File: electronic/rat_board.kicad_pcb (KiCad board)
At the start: 2 copper layers, 44.5 x 49.5 mm, 52 parts, among them P1 FRONT_LEFT_IR, P2 SIDE_LEFT_IR, P3 SIDE_RIGHT_IR, P4 FRONT_RIGHT_IR, P5 LEFT_MOTOR, P6 RIGHT_MOTOR, P7 JTAG, SW1 SW_PUSH_SMALL_H, SW2 SWITCH_INV, SW3 SELECT_BUTTON, SW4 START_BUTTON, U1 TR05S3V3, U2 TB6612FNG, U3 STM32F103C8T6, Y1 32.768kHz, Y2 8MHz

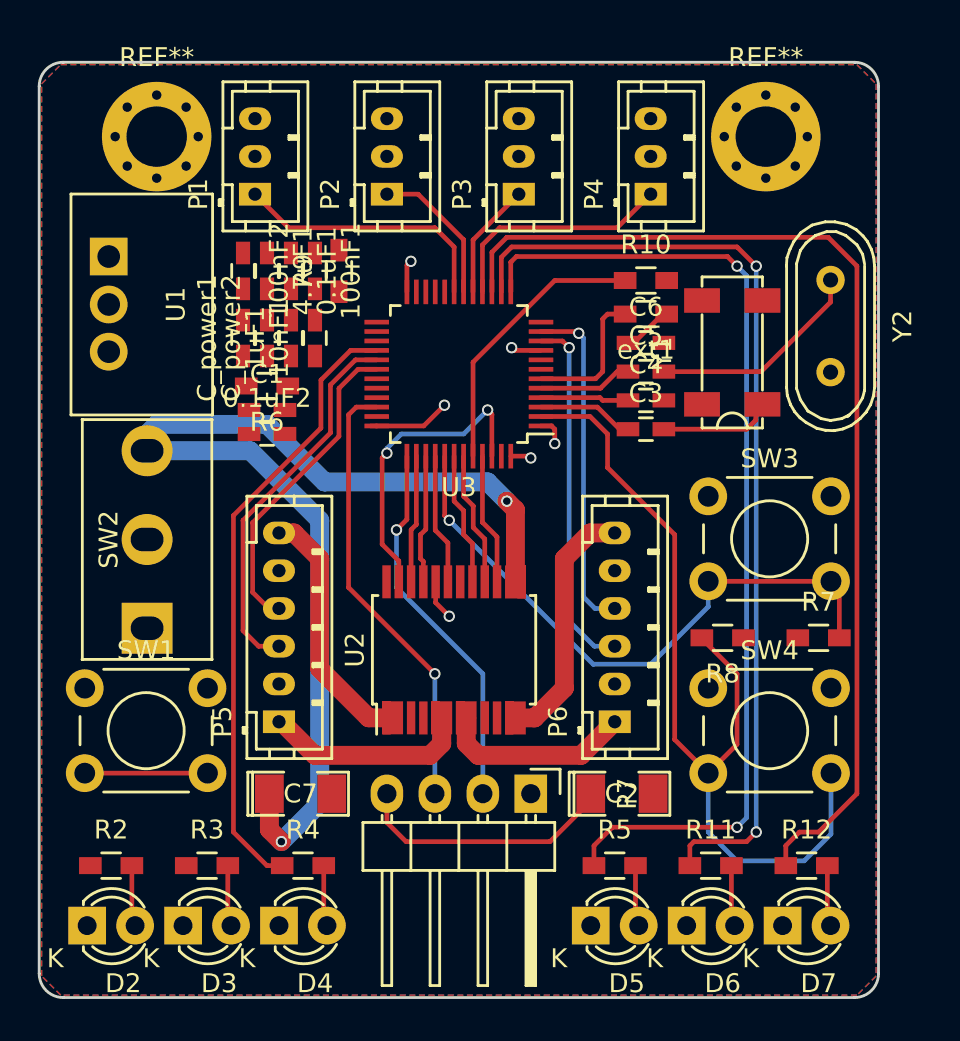
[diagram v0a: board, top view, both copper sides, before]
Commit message: updated pcb
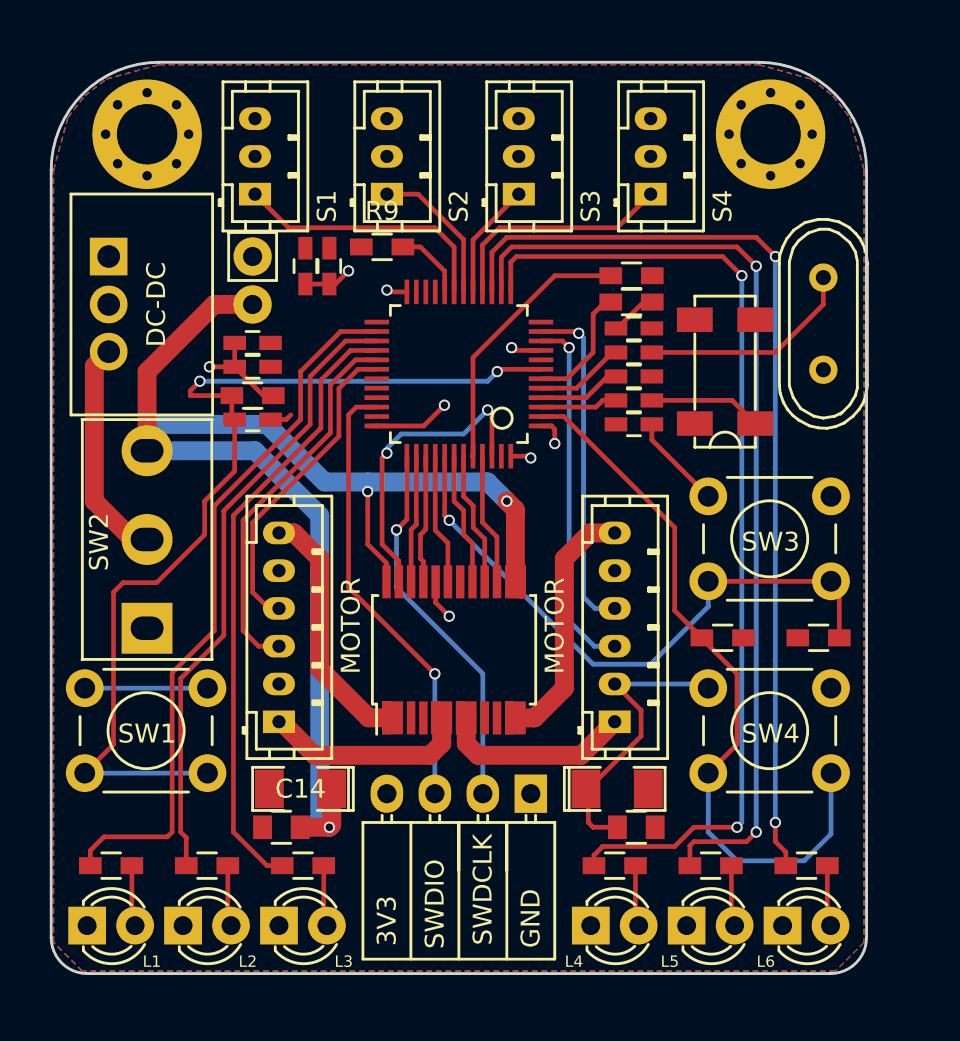
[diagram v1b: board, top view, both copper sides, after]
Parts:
- removed 0.1uF1, 0.1uF2, 100nF1, 100nF2, 10nF1, 1uF1, 4.7uF1, C1, C_power1, C_power2: C, Capacitors_SMD:C_0603_HandSoldering
- removed C2, C7: 10uF, SMD_Packages:SMD-1206_Pol
- removed C3, C4, C5, C6: 20p, Capacitors_SMD:C_0603_HandSoldering
- removed U1: TR05S3V3, Connect:Wafer_Vertical10x5.8x7RM2.5-3
- removed ext1: R, Resistors_SMD:R_0603_HandSoldering
- added ?: 20p, Capacitors_SMD:C_0603_HandSoldering, F.Cu at (65.9, 43.2)
- added ?: 20p, Capacitors_SMD:C_0603_HandSoldering, F.Cu at (65.9, 47.0)
- added ?: 20p, Capacitors_SMD:C_0603_HandSoldering, F.Cu at (65.9, 45.7)
- added ?: 10uF, SMD_Packages:SMD-1206_Pol, F.Cu at (65.0, 67.6)
- added ?: C, Capacitors_SMD:C_0603_HandSoldering, F.Cu at (45.7, 48.0)
- added ?: 100nF, Capacitors_SMD:C_0603_HandSoldering, F.Cu at (45.7, 45.2)
- added ?: 100nF, Capacitors_SMD:C_0603_HandSoldering, F.Cu at (45.7, 43.9)
- added ?: 4.7uF, Capacitors_SMD:C_0603_HandSoldering, F.Cu at (65.9, 48.3)
- added ?: 10nF, Capacitors_SMD:C_0603_HandSoldering, F.Cu at (49.8, 39.9)
- added ?: 1uF, Capacitors_SMD:C_0603_HandSoldering, F.Cu at (48.5, 39.9)
- added ?: 20p, Capacitors_SMD:C_0603_HandSoldering, F.Cu at (65.9, 44.5)
- added ?: R, Resistors_SMD:R_0603_HandSoldering, F.Cu at (65.8, 41.8)
- added ?: 0.1uF, Capacitors_SMD:C_0805, F.Cu at (47.2, 69.6)
- added ?: 0.1uF, Capacitors_SMD:C_0805, F.Cu at (66.0, 69.6)
- added ?: TR05S3V3, custom-lib:TR05S3V3, F.Cu at (38.1, 41.9)
- added C14: 10uF, SMD_Packages:SMD-1206_Pol, F.Cu at (48.3, 67.6)
- added DC-DC: CONN_01X02, Socket_Strips:Socket_Strip_Straight_1x02, F.Cu at (45.7, 41.9)
- moved R9 2.62 mm to (52.6, 38.9), turned to 0 degrees
- moved ? 1.09 mm to (70.7, 45.5)
- moved ? 0.92 mm to (45.7, 46.7)
- moved ? 0.80 mm to (65.8, 40.4)
- moved ? 0.52 mm to (40.1, 32.9)
- moved ? 0.40 mm to (75.9, 42.9)
- moved ? 0.28 mm to (73.2, 32.9)
- renumbered P7 to ?, R3 to ?, R4 to ?, R5 to ?, R7 to ?, R8 to ?, R10 to ?, Y2 to ?, R11 to ?, R12 to ?, REF** to ?, U2 to ?, U3 to ?, Y1 to ?, R6 to ?, R2 to ?, D2 to L1, D3 to L2, D4 to L3, D5 to L4, D6 to L5, D7 to L6, P5 to MOTOR, P6 to MOTOR, P1 to S1, P2 to S2, P3 to S3, P4 to S4
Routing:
- net /RESET: track 6.98 -> 52.9 mm, vias 0 -> 2
- net /LED0: track 0.04 -> 37.7 mm
- net /LED1: track 0.59 -> 33.8 mm
- net +BATT: track 57.6 -> 74.7 mm, vias 2 -> 3
- net +3V3: track 26.5 -> 41.3 mm, vias 6 -> 8
- net Net-(SW2-Pad2): track 0.00 -> 11.9 mm
- net /UB_START: track 47.2 -> 39.1 mm
- net GND: track 0.00 -> 8.00 mm
- net /LED5: track 56.3 -> 50.3 mm, vias 0 -> 2
- net /BOOT1: track 0.00 -> 3.84 mm
- net Net-(C6-Pad1): track 2.68 -> 0.00 mm
- net Net-(C8-Pad1): track 0.00 -> 2.50 mm
- net /OSC32IN: track 5.09 -> 4.12 mm
- net /OSCOUT: track 7.51 -> 6.57 mm
- net /LED3: track 53.1 -> 52.4 mm
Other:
- board size 44.5 x 49.5 mm -> 43.2 x 48.3 mm
